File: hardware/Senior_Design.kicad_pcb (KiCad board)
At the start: 4 copper layers, 135.6 x 132 mm, 152 parts, among them J101 Conn_ARM_JTAG_SWD_10, J201 54-00125, J202 Conn_01x03, J301 Conn_ARM_JTAG_SWD_10, J501 2305018-2, J601 J0011D21BNL, Q201 CSD87503Q3E, Q202 Q_NMOS, Q203 CSD87503Q3E, SW101 SW_Push, SW201 SW_Push, SW301 SW_Push, U101 EFR32FG28A122F1024GM48-A, U201 BQ25798RQMR, U202 TPS63020DSJR, U301 BDE-MB1352P71UA32, U401 TPS613222ADBVR, U402 BME688, U403 USBLC6-2P6, U501 CP2102N-A02-GQFN20, U502 CDSOT236-0504C, U601 W5500, Y101 LF_Crystal, Y102 ECS-390-CDX-1932, Y601 ECS-250-18-5PX-F-TR

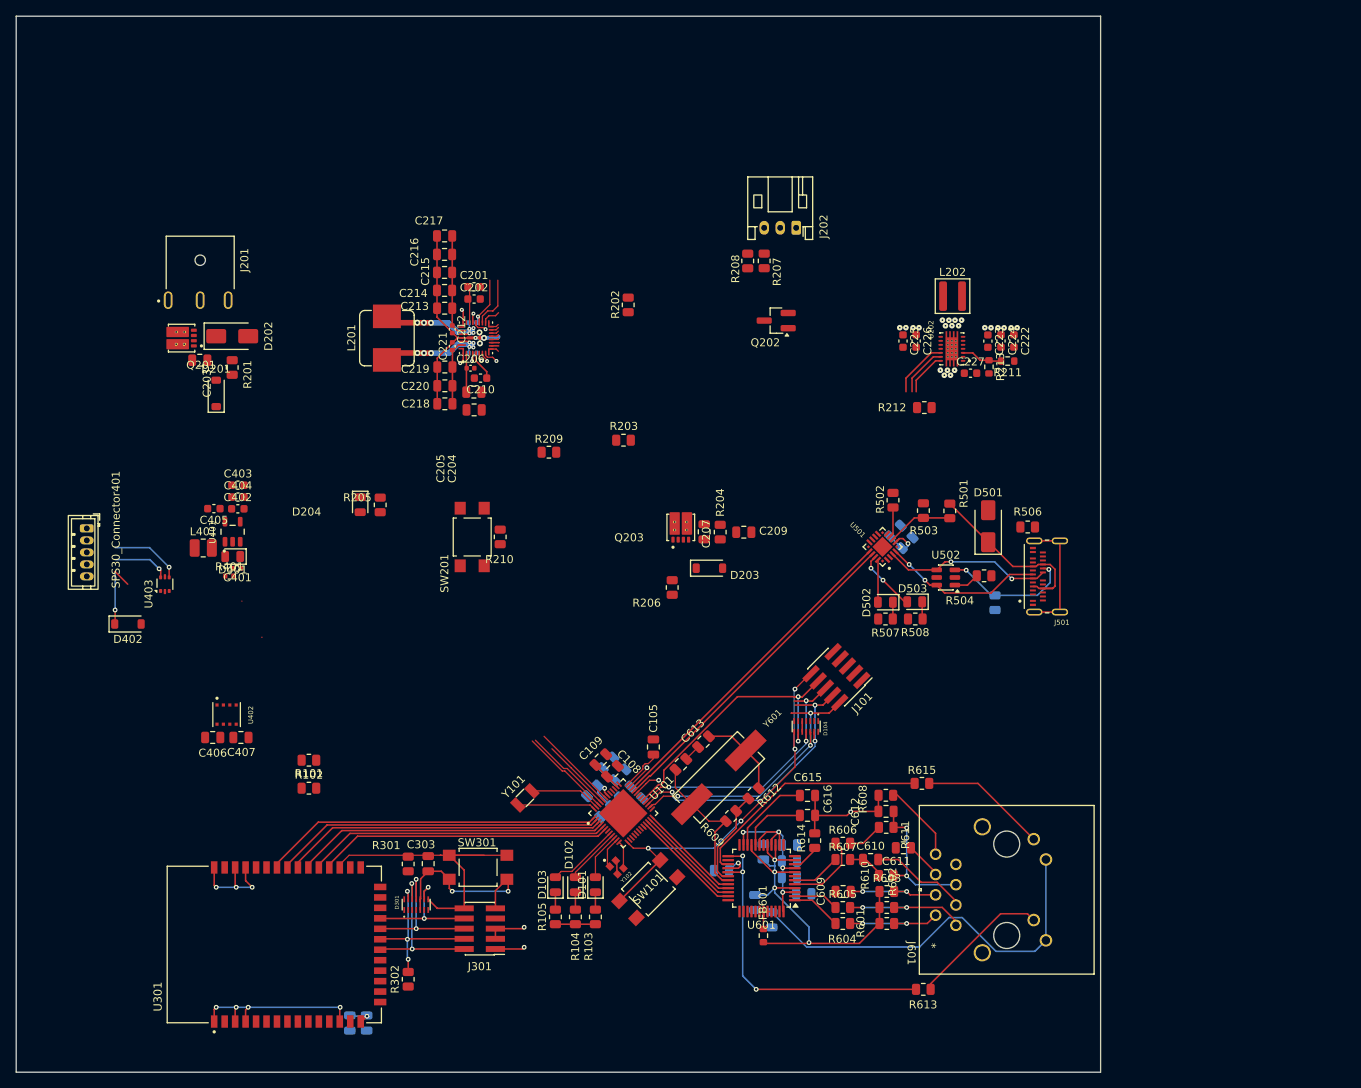
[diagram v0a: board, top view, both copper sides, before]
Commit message: power layout WIP
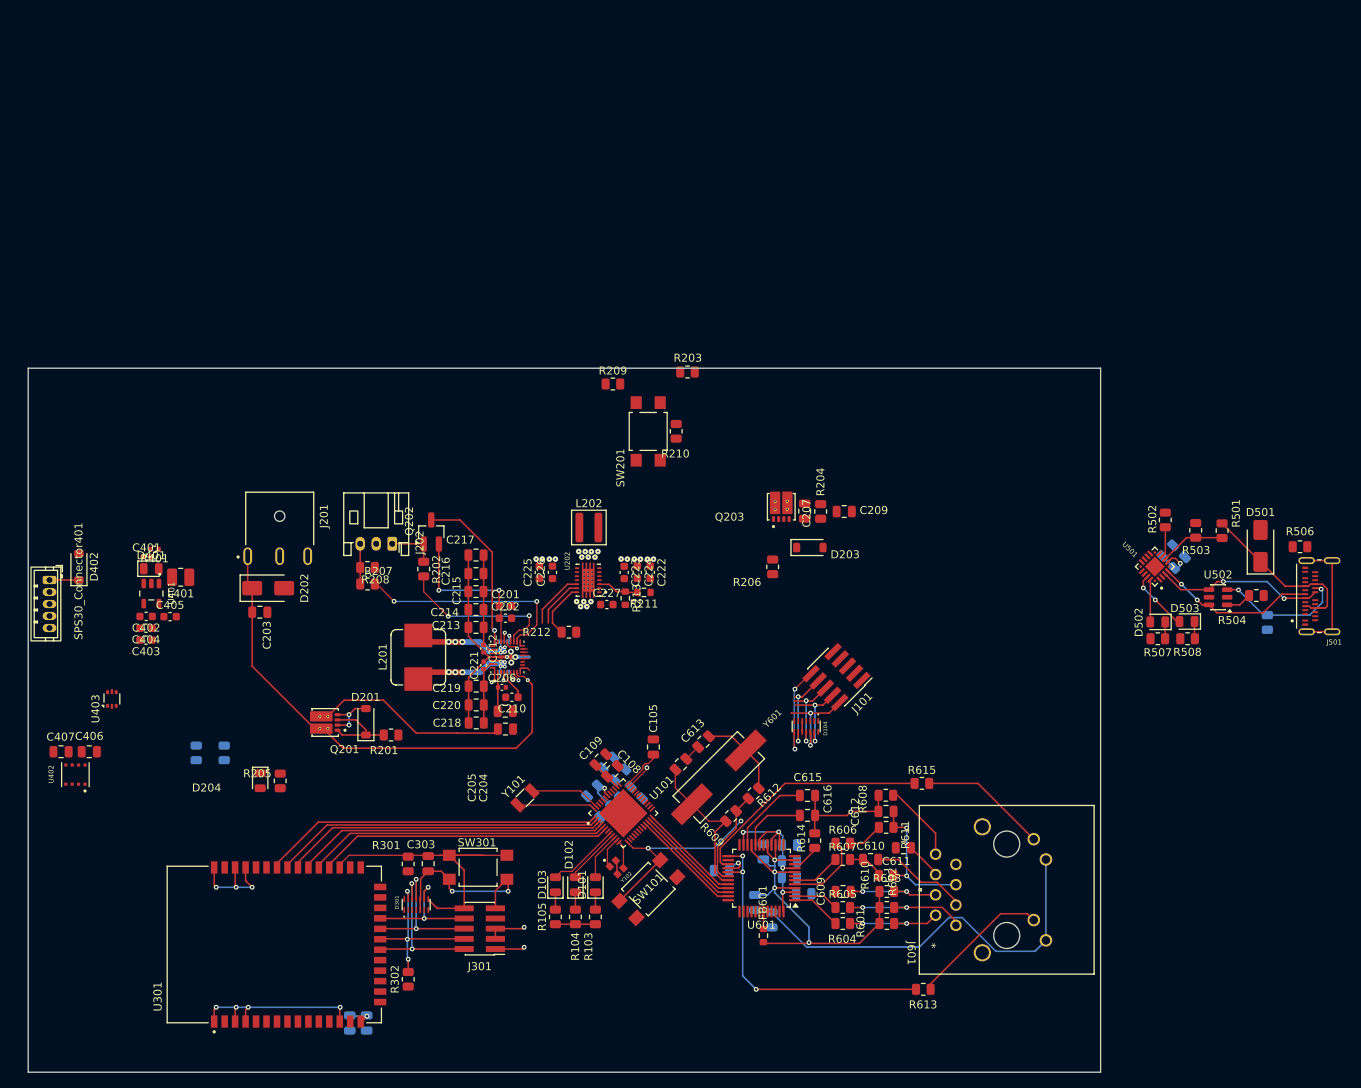
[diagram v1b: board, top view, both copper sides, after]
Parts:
- R101, R102: moved to B.Cu
- moved J202 64.1 mm to (-5.00, -45.0)
- moved R207 63.9 mm to (-8.08, -40.0), turned to 180 degrees
- moved R208 61.1 mm to (-8.09, -42.1), turned to 0 degrees
- moved C227 53.9 mm to (21.8, -37.5)
- moved C224 53.9 mm to (25.6, -41.5)
- moved C222 53.9 mm to (27.3, -41.5)
- moved C223 53.9 mm to (24.0, -41.5)
- moved C225 53.9 mm to (13.4, -41.5), turned to 90 degrees
- moved C226 53.9 mm to (15.0, -41.5), turned to 90 degrees
- moved L202 53.9 mm to (19.6, -47.1)
- moved R211 53.9 mm to (26.5, -39.0)
- moved R213 53.9 mm to (24.1, -38.2)
- moved U202 53.9 mm to (19.5, -40.5)
- moved R212 52.6 mm to (17.1, -34.0)
- moved Q201 51.3 mm to (-13.4, -22.7)
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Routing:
- net /BMS/VAC2: track 1.94 -> 62.7 mm
- net /MCU/MCU_RX_CP_TX: track 42.1 -> 0.00 mm
- net /MCU/MCU_TX_CP_RX: track 42.0 -> 0.00 mm
- net /MCU/JTAG_TCK: track 36.7 -> 10.9 mm, vias 3 -> 2
- net /MCU/JTAG_TDI: track 36.2 -> 10.6 mm
- net /BMS/REGN: track 6.14 -> 31.5 mm, vias 0 -> 2
- net Net-(C204-Pad1): track 4.89 -> 29.4 mm
- net /MCU/JTAG_TDO: track 34.3 -> 10.8 mm, vias 3 -> 2
- net /MCU/JTAG_TMS: track 36.8 -> 13.5 mm, vias 3 -> 2
- net Net-(Q202-G): track 1.71 -> 20.7 mm
- net BAT: track 4.57 -> 19.9 mm, vias 0 -> 2
- net Net-(U201-BATP): track 6.51 -> 20.9 mm, vias 0 -> 2
- net /BME 688 and SPS30/SCL: track 12.6 -> 0.65 mm
- net /BME 688 and SPS30/SDA: track 12.5 -> 0.66 mm
- net /MCU/nRST: track 49.6 -> 37.8 mm
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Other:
- board size 135.6 x 132 mm -> 134.1 x 88 mm
